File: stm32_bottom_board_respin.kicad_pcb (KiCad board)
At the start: 2 copper layers, 90 x 60 mm, 50 parts, among them J1 Conn_01x02, J2 WS2812, J3 FAN_PWM, J4 SSR, J5 PURFUME, J6 Conn_01x14, J7 Conn_01x12, J8 Conn_01x12, Q1 2N3904(1AM), Q2 SS9013_J3, Q3 SS9013_J3, SW1 SW_Push, U2 S102S01, U3 STM32F103C8T6, U4 AMS1117-3.3, Y1 O8M, Y2 O32.768K

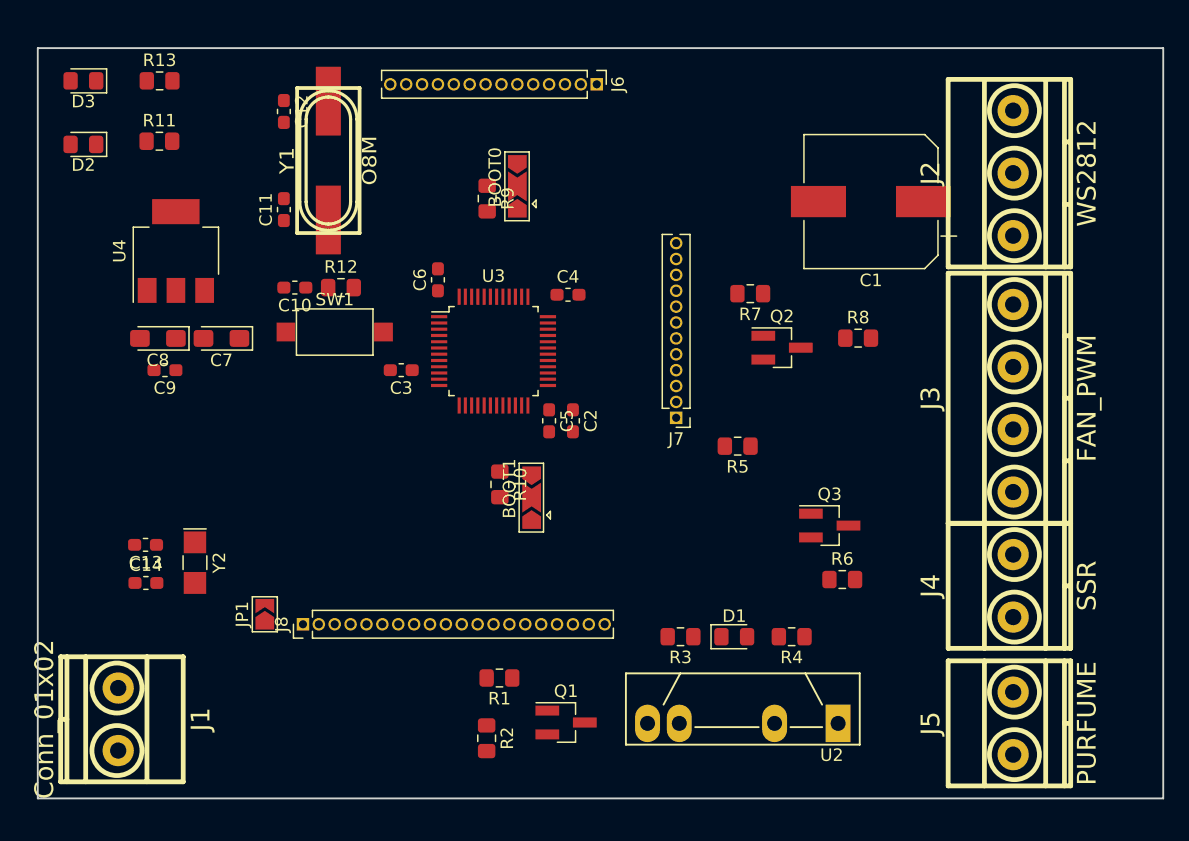
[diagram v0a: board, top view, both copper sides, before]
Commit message: update,
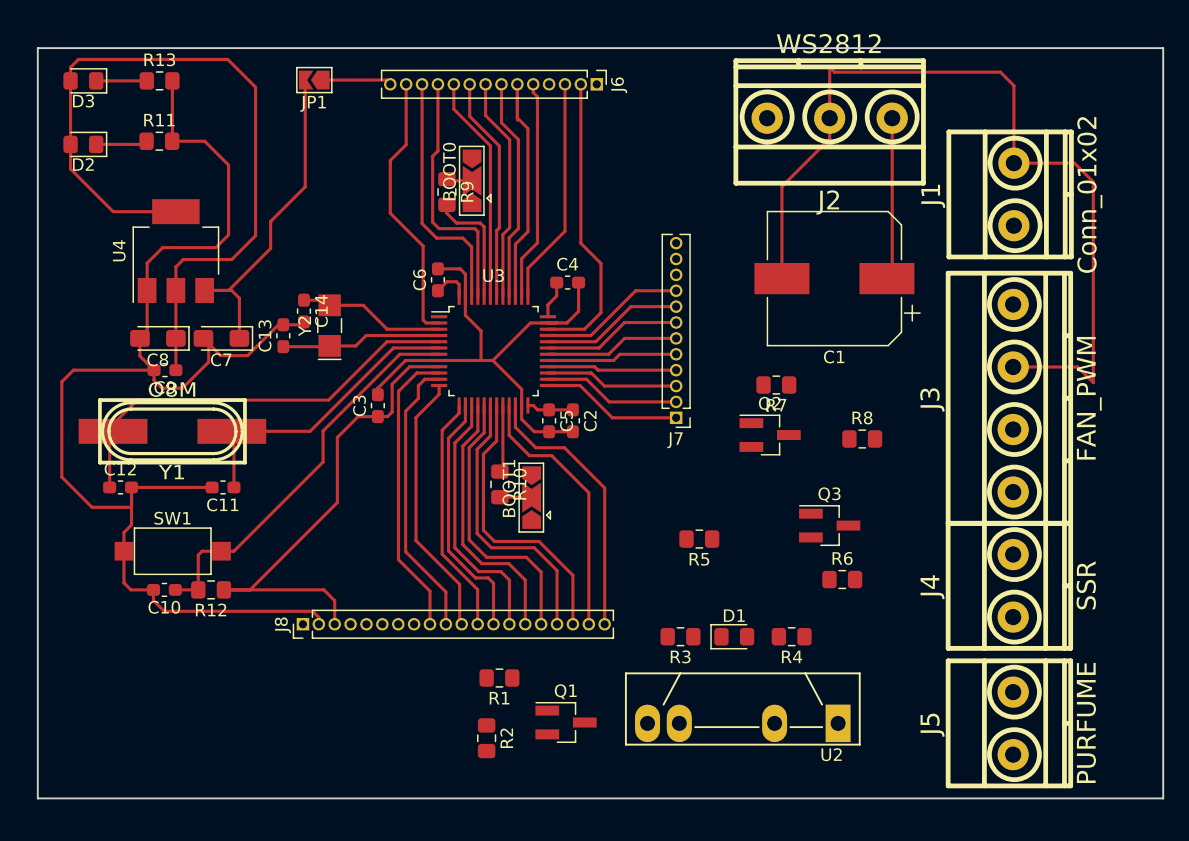
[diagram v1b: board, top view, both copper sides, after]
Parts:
- moved J1 83.0 mm to (83.1, 16.7), turned to 90 degrees
- moved JP1 42.9 mm to (27.1, 7.56), turned to 180 degrees
- moved C12 32.8 mm to (11.6, 40.1), turned to 0 degrees
- moved C10 26.3 mm to (15.1, 48.3)
- moved R12 26.3 mm to (18.9, 48.3), turned to 180 degrees
- moved C14 25.1 mm to (26.3, 26.0), turned to 270 degrees
- moved Y1 25.0 mm to (15.8, 35.6), turned to 180 degrees
- moved C11 22.7 mm to (19.8, 40.1), turned to 180 degrees
- moved Y2 21.8 mm to (28.3, 27.2), turned to 90 degrees
- moved SW1 21.8 mm to (15.8, 45.2)
- moved C13 20.0 mm to (24.6, 28.0), turned to 90 degrees
- moved J2 15.3 mm to (68.3, 10.6), turned to 180 degrees
- moved R8 8.07 mm to (70.9, 36.3)
- moved R5 8.04 mm to (57.9, 44.3)
- moved R7 7.59 mm to (64.1, 31.9)
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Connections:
- J6 pad 13: Net-(J6-Pad13) -> /STM32_CORE/PC13
- J6 pad 14: /STM32_CORE/PC13 -> Net-(J6-Pad14)
- JP1 pad 1: Net-(J8-Pad1) -> Net-(J6-Pad14)
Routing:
- net GND: track 0.00 -> 218.4 mm
- net +3V3: track 0.00 -> 111.4 mm
- net /STM32_CORE/OSCIN: track 0.00 -> 34.0 mm
- net /STM32_CORE/RESET: track 0.00 -> 32.0 mm
- net +5V: track 0.00 -> 27.5 mm
- net /STM32_CORE/OSCOUT: track 0.00 -> 23.9 mm
- net /STM32_CORE/SWIO: track 0.00 -> 23.7 mm
- net /STM32_CORE/PA0: track 0.00 -> 23.5 mm
- net /STM32_CORE/PB1: track 0.00 -> 23.0 mm
- net /STM32_CORE/PA1: track 0.00 -> 22.7 mm
- net /STM32_CORE/PB0: track 0.00 -> 22.6 mm
- net /STM32_CORE/PA7: track 0.00 -> 22.2 mm
- net /STM32_CORE/PC13: track 0.00 -> 21.8 mm
- net /STM32_CORE/PB11: track 0.00 -> 21.8 mm
- net /STM32_CORE/PA2: track 0.00 -> 21.4 mm
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
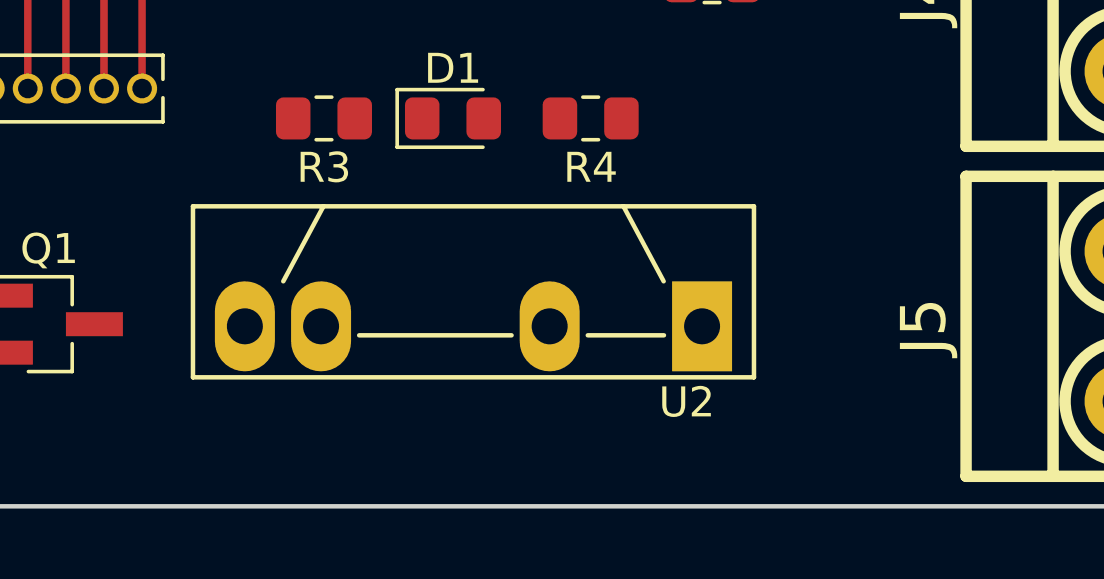
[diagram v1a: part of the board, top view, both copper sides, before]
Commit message: update,
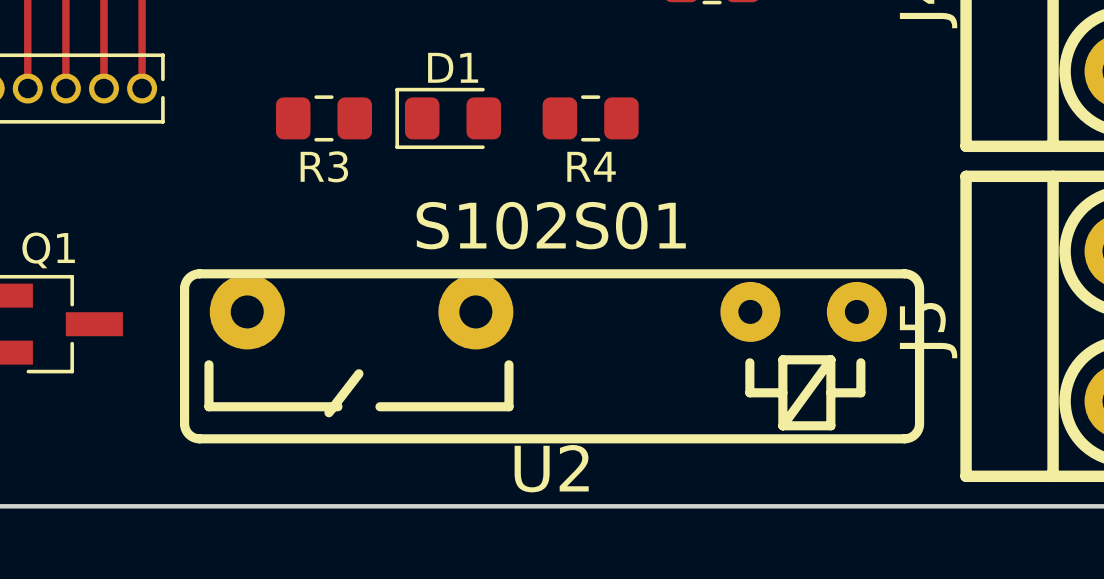
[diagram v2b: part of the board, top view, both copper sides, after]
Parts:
- U2: footprint Package_SIP:SIP4_Sharp-SSR_P7.62mm_Straight -> footprint-lib:OMRON-G3MB-202P
- moved U2 5.10 mm to (64.0, 60.0)
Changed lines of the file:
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@@
     (add_net VWS2812)
+  )
+  (module footprint-lib:OMRON-G3MB-202P (layer F.Cu)
+    (at 64 60 180)
+    (descr "relay, 34.51series")
+    (fp_text reference U2 (at 0 -3.8 180) (layer F.SilkS)
+      (effects (font (size 1.524 1.524) (thickness 0.3048)))
+    )
+    (fp_text value S102S01 (at 0 4.3 180) (layer F.SilkS)
+      (effects (font (size 1.524 1.524) (thickness 0.3048)))
+    )
+    (fp_arc (start 11.74962 -2.24962) (end 11.74962 -2.75) (angle 90) (layer F.SilkS) (width 0.3048))
+    (fp_arc (start -11.74962 -2.24962) (end -12.25 -2.24962) (angle 90) (layer F.SilkS) (width 0.3048))
+    (fp_line (start -11.74962 -2.75) (end 11.74962 -2.75) (layer F.SilkS) (width 0.3048))
+    (fp_line (start -11.74962 2.75) (end 11.74962 2.75) (layer F.SilkS) (width 0.3048))
+    (fp_line (start -12.25 -2.24962) (end -12.25 2.24962) (layer F.SilkS) (width 0.3048))
+    (fp_line (start 12.25 -2.24962) (end 12.25 2.24962) (layer F.SilkS) (width 0.3048))
+    (fp_line (start 11.437241 -0.281265) (end 11.437241 -1.681265) (layer F.SilkS) (width 0.3048))
+    (fp_line (start 6.437241 -0.581265) (end 7.437241 -1.881265) (layer F.SilkS) (width 0.3048))
+    (fp_line (start 11.437241 -1.681265) (end 7.137241 -1.681265) (layer F.SilkS) (width 0.3048))
+    (fp_line (start 5.737241 -1.681265) (end 1.437241 -1.681265) (layer F.SilkS) (width 0.3048))
+    (fp_line (start 1.437241 -0.281265) (end 1.437241 -1.681265) (layer F.SilkS) (width 0.3048))
+    (fp_line (start -9.293278 -2.316312) (end -9.293278 -0.116312) (layer F.SilkS) (width 0.3048))
+    (fp_line (start -7.693278 -2.316312) (end -9.293278 -2.316312) (layer F.SilkS) (width 0.3048))
+    (fp_line (start -7.693278 -0.116312) (end -7.693278 -2.316312) (layer F.SilkS) (width 0.3048))
+    (fp_line (start -9.293278 -0.116312) (end -7.693278 -0.116312) (layer F.SilkS) (width 0.3048))
+    (fp_line (start -7.693278 -2.316312) (end -9.293278 -0.116312) (layer F.SilkS) (width 0.3048))
+    (fp_line (start -7.693278 -1.216312) (end -6.593278 -1.216312) (layer F.SilkS) (width 0.3048))
+    (fp_line (start -9.293278 -1.216312) (end -10.293278 -1.216312) (layer F.SilkS) (width 0.3048))
+    (fp_line (start -6.593278 -0.216312) (end -6.593278 -1.216312) (layer F.SilkS) (width 0.3048))
+    (fp_line (start -10.293278 -0.216312) (end -10.293278 -1.216312) (layer F.SilkS) (width 0.3048))
+    (fp_arc (start 11.74962 2.24962) (end 12.25 2.24962) (angle 90) (layer F.SilkS) (width 0.3048))
+    (fp_arc (start -11.74962 2.24962) (end -11.74962 2.75) (angle 90) (layer F.SilkS) (width 0.3048))
+    (pad 2 thru_hole circle (at 2.54 1.48 180) (size 2.5 2.5) (drill 1.1) (layers *.Cu *.Mask)
+      (net 23 /SSR_CH1_OUTPUT1))
+    (pad 4 thru_hole circle (at -10.16 1.48 180) (size 2 2) (drill 0.8) (layers *.Cu *.Mask)
+      (net 16 "Net-(Q1-Pad3)"))
+    (pad 1 thru_hole circle (at 10.16 1.48 180) (size 2.5 2.5) (drill 1.1) (layers *.Cu *.Mask)
+      (net 22 /SSR_CH1_OUTPUT2))
+    (pad 3 thru_hole circle (at -6.61 1.48 180) (size 2 2) (drill 0.8) (layers *.Cu *.Mask)
+      (net 15 "Net-(R4-Pad2)"))
   )
   (module w_conn_mkds:mkds_1,5-2 (layer F.Cu)
@@
       (net 18 +3V3))
     (model ${KISYS3DMOD}/Package_QFP.3dshapes/LQFP-48_7x7mm_P0.5mm.wrl
-      (at (xyz 0 0 0))
-      (scale (xyz 1 1 1))
-      (rotate (xyz 0 0 0))
-    )
-  )
-  (module Package_SIP:SIP4_Sharp-SSR_P7.62mm_Straight (layer F.Cu)
-    (at 69 59 180)
-    (descr "SIP4 Footprint for SSR made by Sharp")
-    (tags "Solid State relais SSR Sharp")
-    (fp_text reference U2 (at 0.508 -2.54 180) (layer F.SilkS)
-      (effects (font (size 1 1) (thickness 0.15)))
-    )
-    (fp_text value S102S01 (at 7.62 5 180) (layer F.Fab)
-      (effects (font (size 1 1) (thickness 0.15)))
-    )
-    (fp_text user %R (at 7.62 0 180) (layer F.Fab)
-      (effects (font (size 1 1) (thickness 0.15)))
-    )
-    (fp_line (start 1.27 -0.3) (end 3.81 -0.3) (layer F.SilkS) (width 0.15))
-    (fp_line (start 6.35 -0.3) (end 11.43 -0.3) (layer F.SilkS) (width 0.15))
-    (fp_line (start 17.25 -1.95) (end 17.25 4.25) (layer F.CrtYd) (width 0.05))
-    (fp_line (start 17.25 4.25) (end -2 4.25) (layer F.CrtYd) (width 0.05))
-    (fp_line (start -2 4.25) (end -2 -1.95) (layer F.CrtYd) (width 0.05))
-    (fp_line (start -2 -1.95) (end 17.25 -1.95) (layer F.CrtYd) (width 0.05))
-    (fp_line (start 2.62 4) (end 1.28 1.5) (layer F.SilkS) (width 0.15))
-    (fp_line (start 12.62 4) (end 13.96 1.5) (layer F.SilkS) (width 0.15))
-    (fp_line (start -1.73 -1.7) (end 16.97 -1.7) (layer F.SilkS) (width 0.15))
-    (fp_line (start 16.97 -1.7) (end 16.97 4) (layer F.SilkS) (width 0.15))
-    (fp_line (start 16.97 4) (end -1.73 4) (layer F.SilkS) (width 0.15))
-    (fp_line (start -1.73 4) (end -1.73 -1.7) (layer F.SilkS) (width 0.15))
-    (fp_line (start -1.6 3.9) (end 16.8 3.9) (layer F.Fab) (width 0.1))
-    (fp_line (start 16.8 3.9) (end 16.8 -1.6) (layer F.Fab) (width 0.1))
-    (fp_line (start 16.8 -1.6) (end -0.6 -1.6) (layer F.Fab) (width 0.1))
-    (fp_line (start -0.6 -1.6) (end -1.6 -0.6) (layer F.Fab) (width 0.1))
-    (fp_line (start -1.6 -0.6) (end -1.6 3.9) (layer F.Fab) (width 0.1))
-    (pad 1 thru_hole rect (at 0 0 180) (size 2 3) (drill 1.2) (layers *.Cu *.Mask)
-      (net 22 /SSR_CH1_OUTPUT2))
-    (pad 2 thru_hole oval (at 5.08 0 180) (size 2 3) (drill 1.2) (layers *.Cu *.Mask)
-      (net 23 /SSR_CH1_OUTPUT1))
-    (pad 3 thru_hole oval (at 12.7 0 180) (size 2 3) (drill 1.2) (layers *.Cu *.Mask)
-      (net 15 "Net-(R4-Pad2)"))
-    (pad 4 thru_hole oval (at 15.24 0 180) (size 2 3) (drill 1.2) (layers *.Cu *.Mask)
-      (net 16 "Net-(Q1-Pad3)"))
-    (model ${KISYS3DMOD}/Package_SIP.3dshapes/SIP4_Sharp-SSR_P7.62mm_Straight.wrl
       (at (xyz 0 0 0))
       (scale (xyz 1 1 1))
@@
   (segment (start 20.261497 24.379003) (end 23.622 21.0185) (width 0.25) (layer F.Cu) (net 6))
   (segment (start 18.344088 24.379003) (end 20.261497 24.379003) (width 0.25) (layer F.Cu) (net 6))
-  (segment (start 28.177003 7.894003) (end 27.8395 7.5565) (width 0.25) (layer F.Cu) (net 76))
   (segment (start 44.460088 40.914003) (end 44.492088 40.946003) (width 0.25) (layer F.Cu) (net 7) (status 30))
   (segment (start 41.952088 40.914003) (end 44.460088 40.914003) (width 0.25) (layer F.Cu) (net 7) (status 30))
@@
   (segment (start 37.843503 15.609503) (end 37.719 15.485) (width 0.25) (layer F.Cu) (net 75) (status 30))
   (segment (start 39.729588 15.609503) (end 37.843503 15.609503) (width 0.25) (layer F.Cu) (net 75) (status 30))
+  (segment (start 28.177003 7.894003) (end 27.8395 7.5565) (width 0.25) (layer F.Cu) (net 76))
   (segment (start 32.851585 7.5565) (end 33.189088 7.894003) (width 0.25) (layer F.Cu) (net 76))
   (segment (start 27.8395 7.5565) (end 32.851585 7.5565) (width 0.25) (layer F.Cu) (net 76))
